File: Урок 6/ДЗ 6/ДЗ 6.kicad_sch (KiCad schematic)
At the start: 20 parts, among them SW1 SW_Push

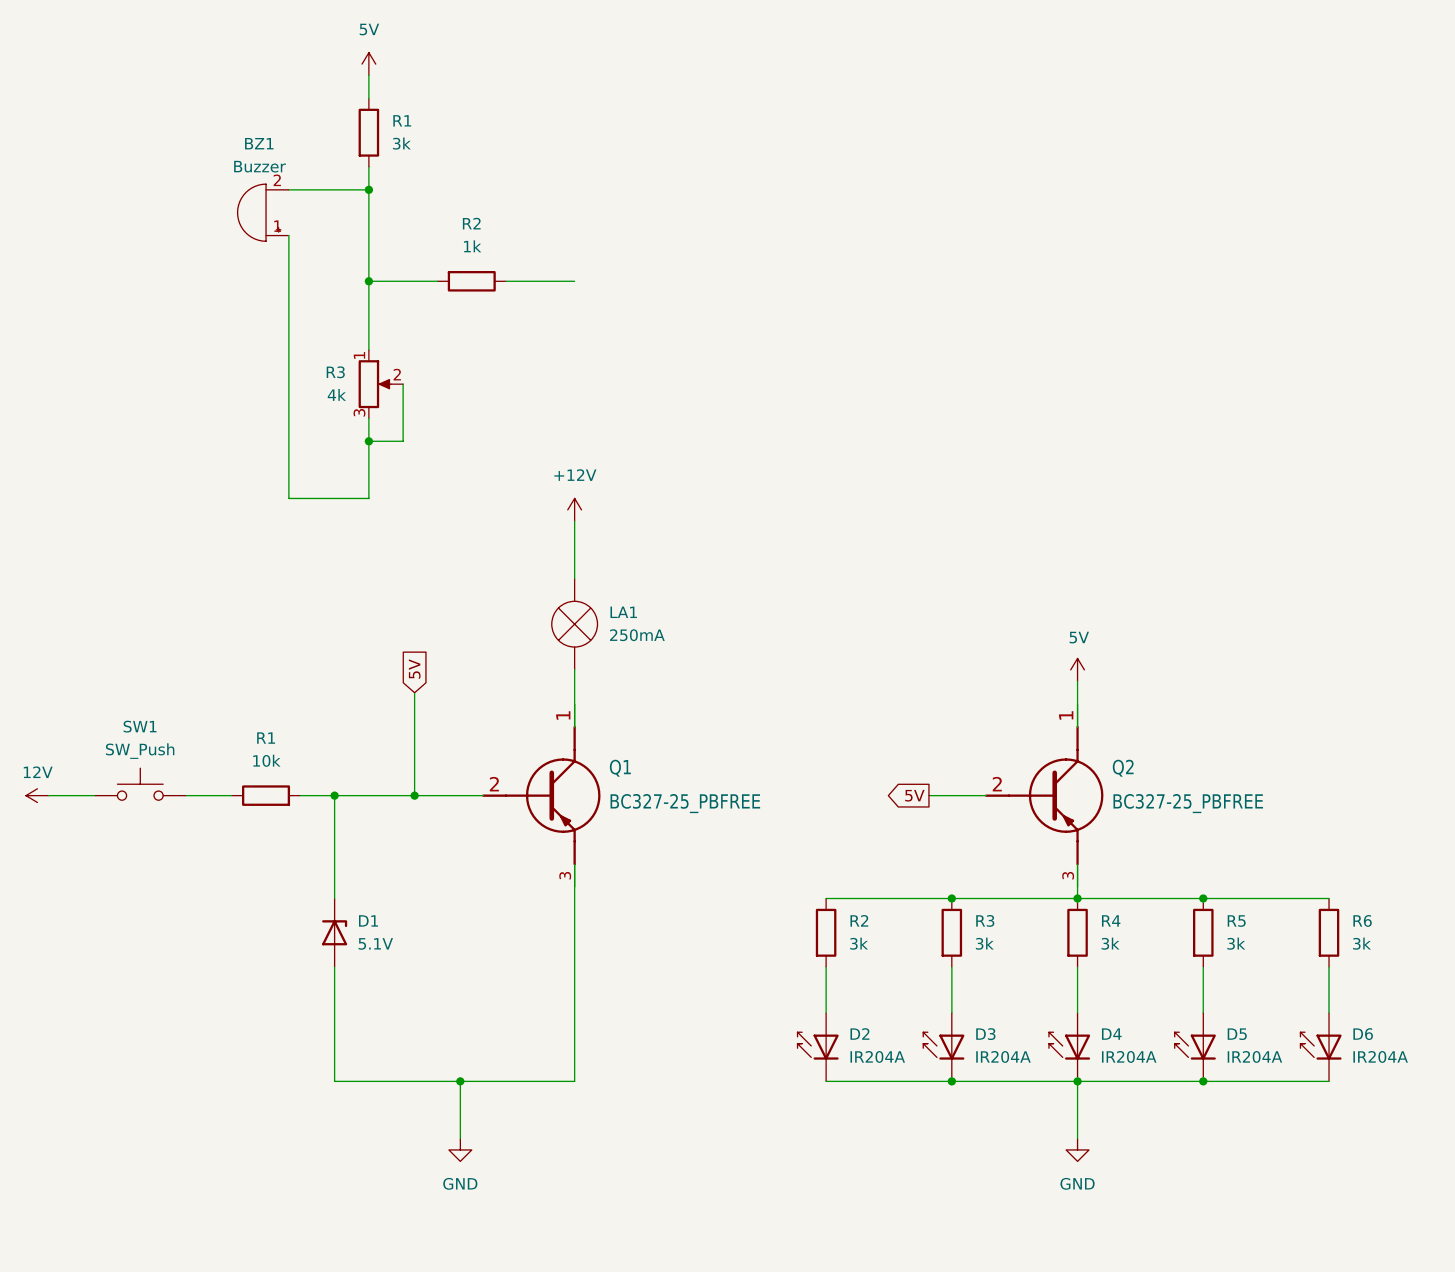
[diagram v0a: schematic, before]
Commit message: 1
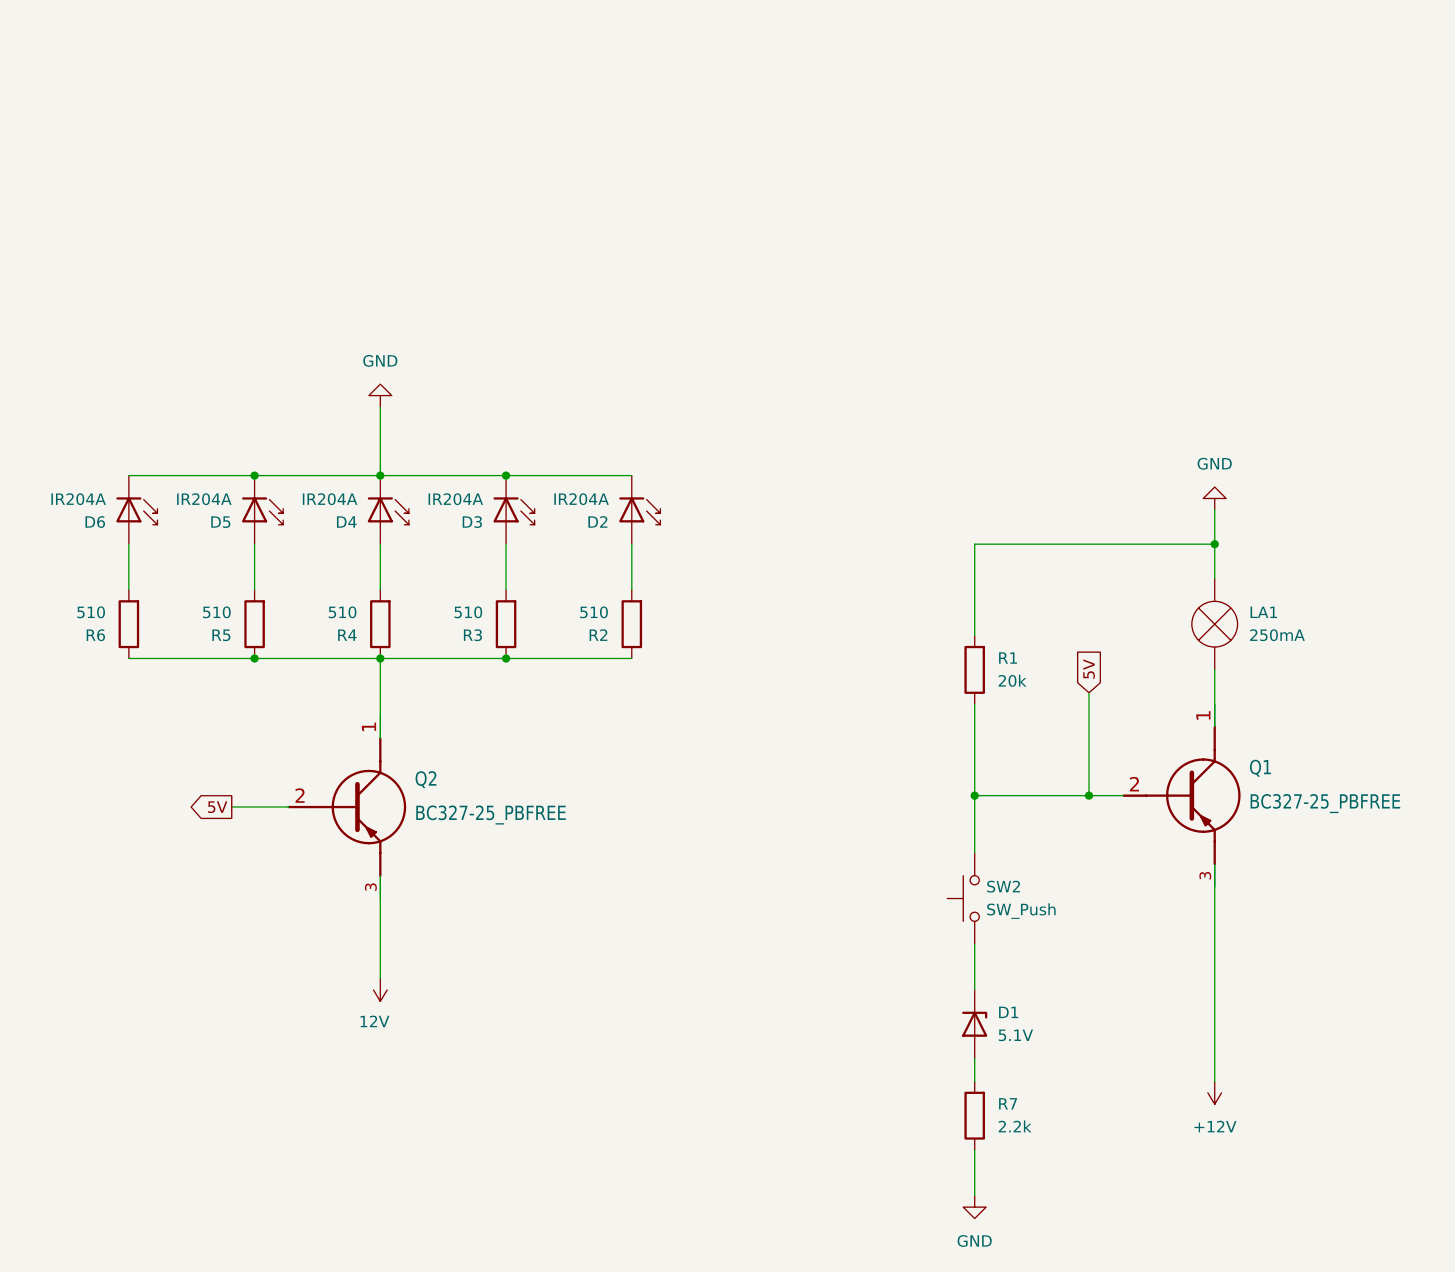
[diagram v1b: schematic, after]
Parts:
- removed BZ1: Buzzer, symbol Device:Buzzer
- removed R1: 3k, symbol Device:R
- removed R2: 1k, symbol Device:R
- removed R3: 4k, symbol Device:R_Potentiometer
- removed SW1: SW_Push, symbol Switch:SW_Push
- added R7: 2.2k, symbol Device:R
- added SW2: SW_Push, symbol Switch:SW_Push
- R1: value 10k -> 20k
- R2, R3, R4, R5, R6: value 3k -> 510
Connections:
- net +12V: now also Q1.3 (A); no longer LA1.2 (+)
- net 12V: now also Q2.3 (A)
- net 5V: now also R1.1, SW2.2; no longer D1.1 (K), Q2.1 (C), R1.2
- net GND: now also LA1.2 (+), R1.2, R7.1; no longer D1.2 (A), Q1.3 (A)
- net at R2.1, R3.1, R4.1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: now also Q2.1 (C); no longer Q2.3 (A)
- new net: D1.1 (K), SW2.1
- new net: D1.2 (A), R7.2
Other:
- moved on the sheet: D1, D2, D3, D4, D5, D6, LA1, Q1, Q2, R1, R2, R3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
